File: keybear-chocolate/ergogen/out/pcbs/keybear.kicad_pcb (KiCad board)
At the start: 2 copper layers, 149.6 x 139.7 mm, 24 parts

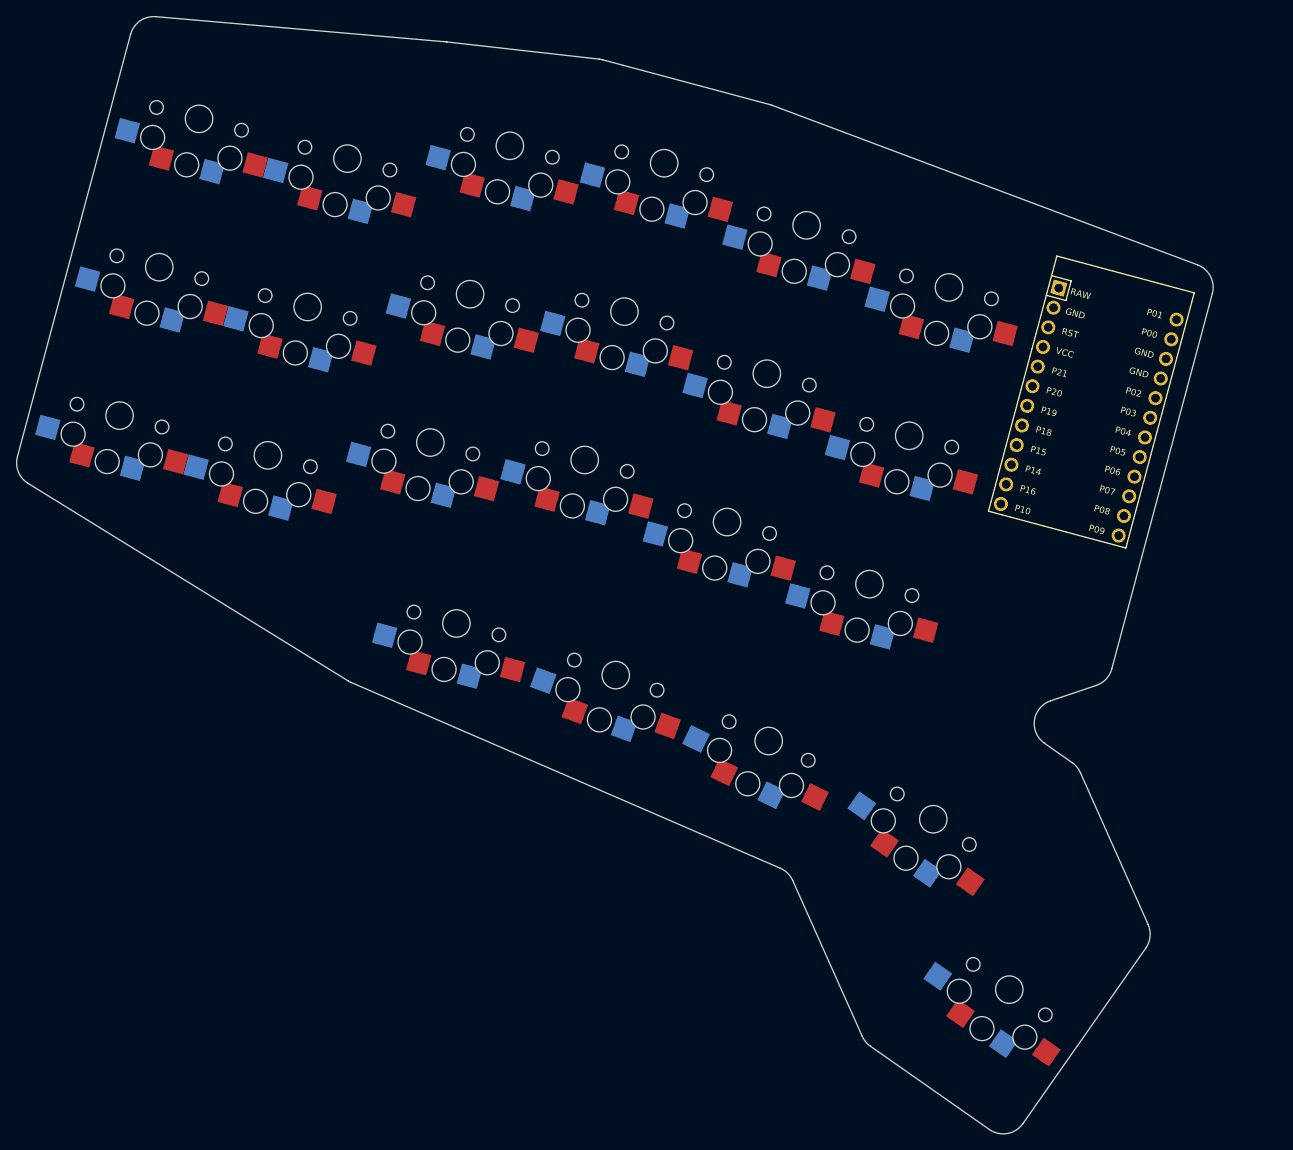
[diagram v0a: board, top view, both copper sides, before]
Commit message: latest ergogen output
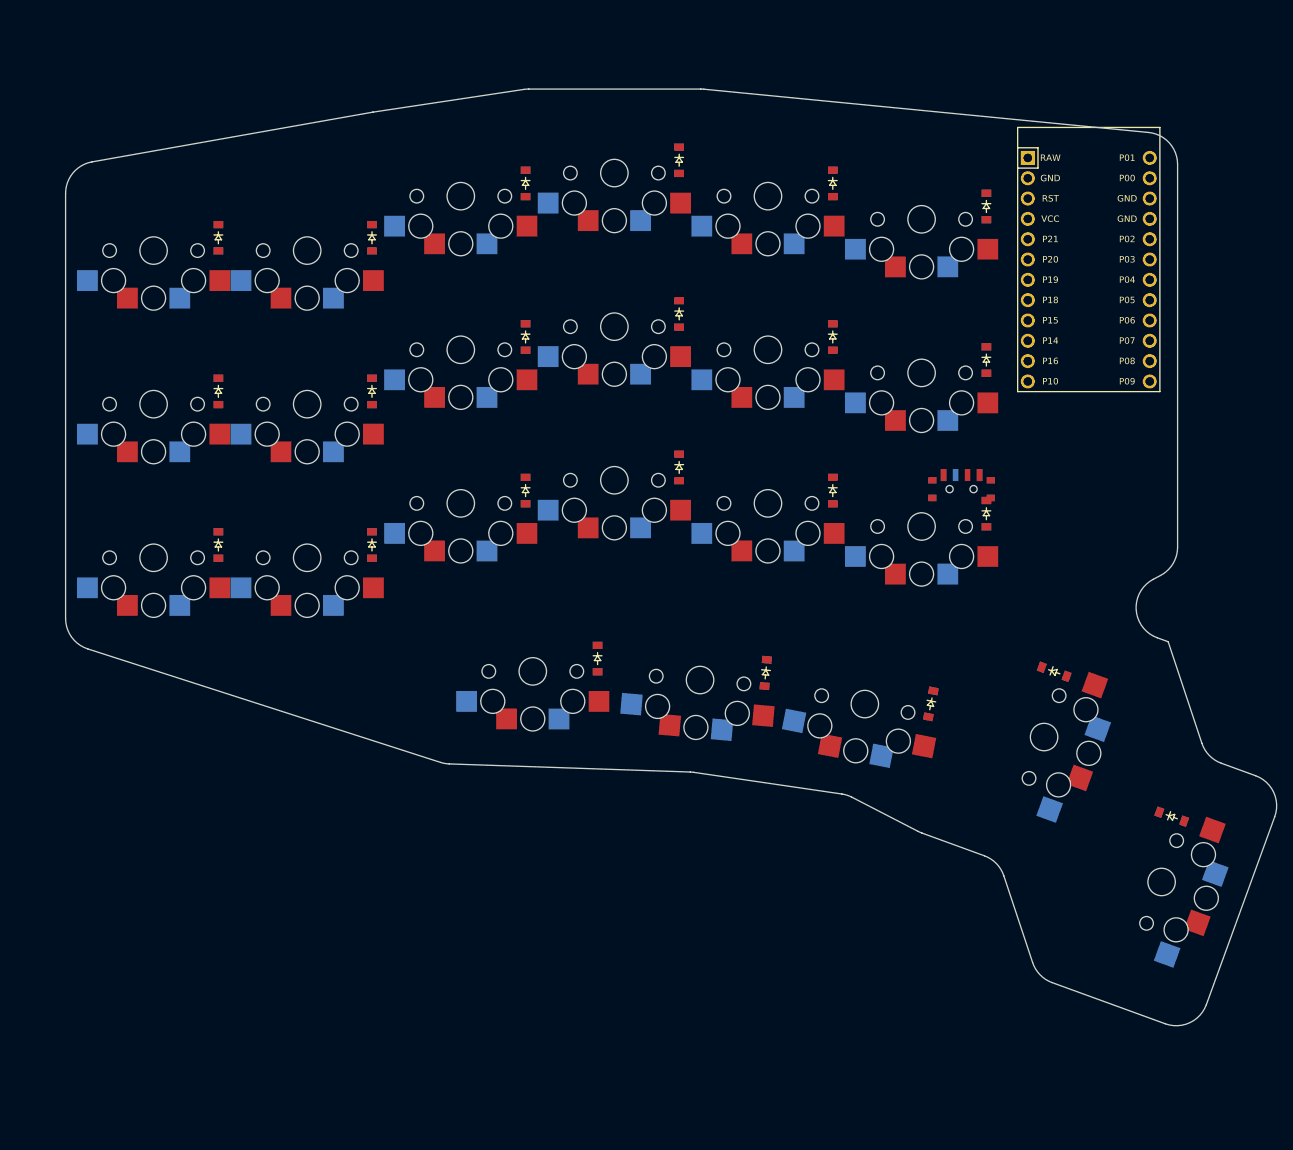
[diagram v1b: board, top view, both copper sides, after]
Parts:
- added ?: , Button_Switch_SMD:SW_SPDT_PCM12, F.Cu at (251.0, 141.1)
- added D1: , ComboDiode, F.Cu at (158.1, 148.4)
- added D10: , ComboDiode, F.Cu at (215.7, 138.7)
- added D11: , ComboDiode, F.Cu at (215.7, 119.5)
- added D12: , ComboDiode, F.Cu at (215.7, 100.3)
- added D13: , ComboDiode, F.Cu at (234.9, 141.6)
- added D14: , ComboDiode, F.Cu at (234.9, 122.4)
- added D15: , ComboDiode, F.Cu at (234.9, 103.2)
- added D16: , ComboDiode, F.Cu at (254.1, 144.5)
- added D17: , ComboDiode, F.Cu at (254.1, 125.3)
- added D18: , ComboDiode, F.Cu at (254.1, 106.1)
- added D19: , ComboDiode, F.Cu at (205.5, 162.6)
- added D2: , ComboDiode, F.Cu at (158.1, 129.2)
- added D20: , ComboDiode, F.Cu at (226.5, 164.4)
- added D21: , ComboDiode, F.Cu at (247.2, 168.3)
- added D22: , ComboDiode, F.Cu at (262.6, 164.3)
- added D23: , ComboDiode, F.Cu at (277.3, 182.4)
- added D3: , ComboDiode, F.Cu at (158.1, 110.0)
- added D4: , ComboDiode, F.Cu at (177.3, 148.4)
- added D5: , ComboDiode, F.Cu at (177.3, 129.2)
- added D6: , ComboDiode, F.Cu at (177.3, 110.0)
- added D7: , ComboDiode, F.Cu at (196.5, 141.6)
- added D8: , ComboDiode, F.Cu at (196.5, 122.4)
- added D9: , ComboDiode, F.Cu at (196.5, 103.2)
- moved S23 23.3 mm to (276.0, 190.5), turned to 250 degrees
- moved S1 18.3 mm to (150.0, 150.0), turned to 180 degrees
- moved MCU1 17.8 mm to (266.9, 114.0), turned to -90 degrees
- moved S3 17.4 mm to (150.0, 111.6), turned to 180 degrees
- moved S22 17.2 mm to (261.3, 172.4), turned to 250 degrees
- moved S2 17.1 mm to (150.0, 130.8), turned to 180 degrees
- moved S4 13.7 mm to (169.2, 150.0), turned to 180 degrees
- moved S21 12.9 mm to (238.9, 168.3), turned to 169 degrees
- moved S6 12.5 mm to (169.2, 111.6), turned to 180 degrees
- moved S5 12.1 mm to (169.2, 130.8), turned to 180 degrees
- moved S19 11.3 mm to (197.4, 164.2), turned to 180 degrees
- moved S20 10.6 mm to (218.3, 165.3), turned to 175 degrees
- moved S16 9.72 mm to (246.0, 146.1), turned to 180 degrees
- moved S18 9.18 mm to (246.0, 107.7), turned to 180 degrees
- moved S9 8.79 mm to (188.4, 104.8), turned to 180 degrees
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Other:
- board size 149.6 x 139.7 mm -> 151.4 x 117.1 mm
